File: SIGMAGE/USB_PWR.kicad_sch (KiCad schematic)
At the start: 45 parts, among them J1 UJ31CHG2SMTTR, U1 MAX8902BATA/V+T, U2 MAX8902BATA/V+T, U3 MAX8902BATA/V+T

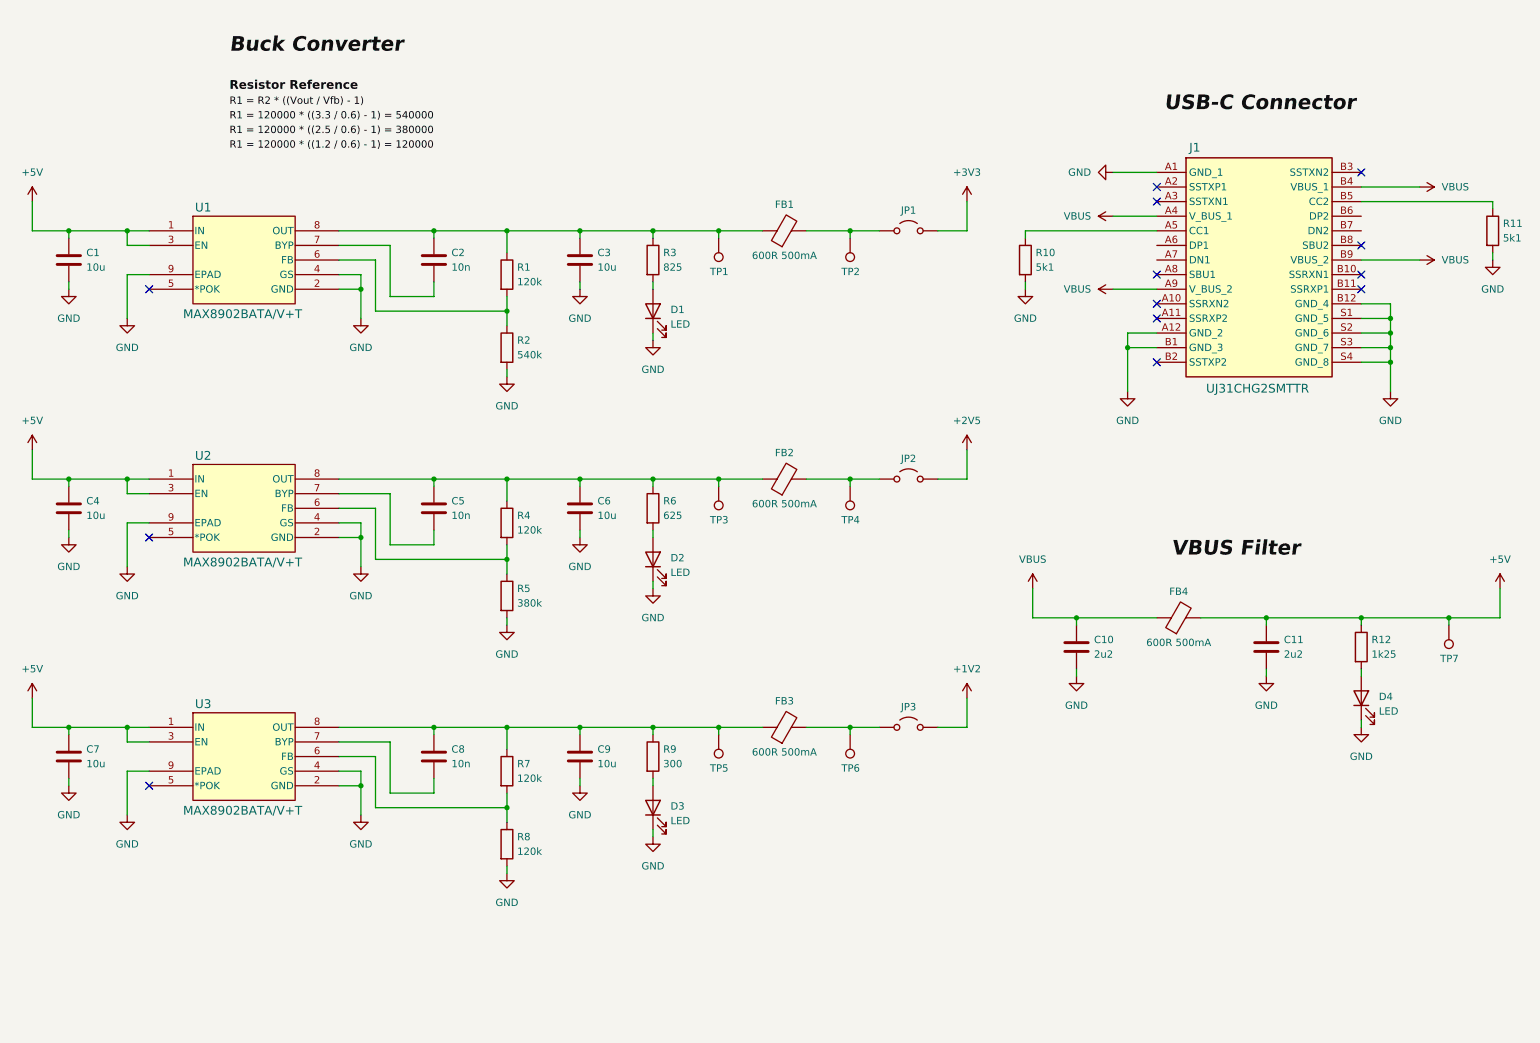
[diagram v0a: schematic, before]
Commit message: Finished schematic
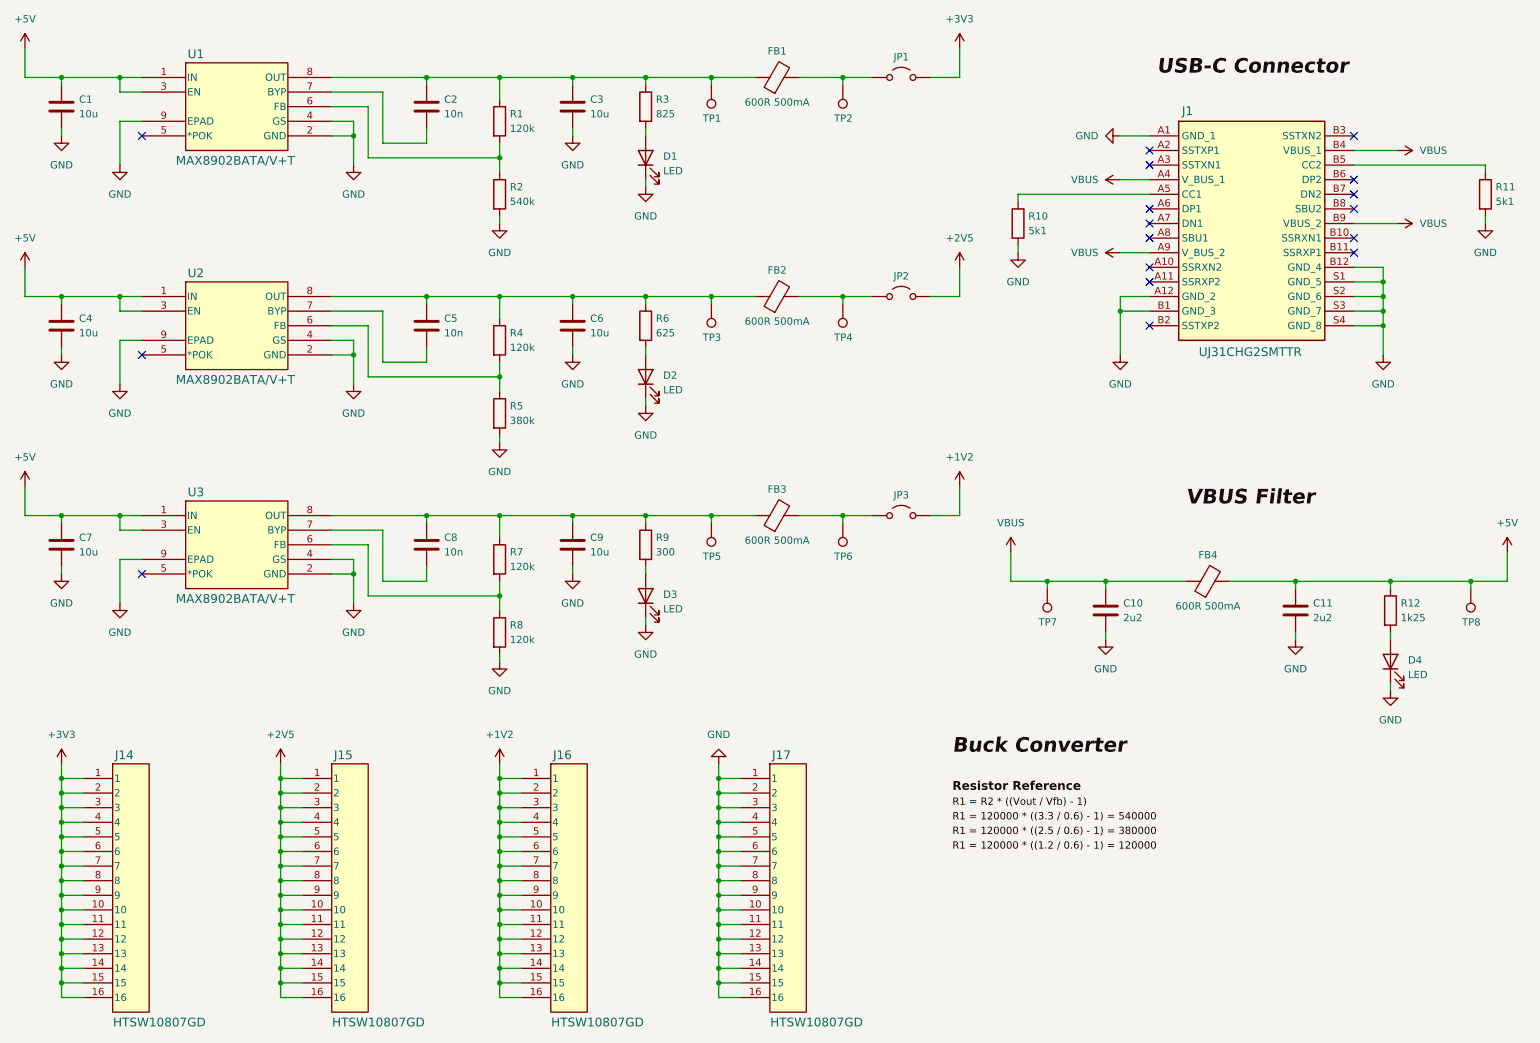
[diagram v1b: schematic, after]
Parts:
- added J14, J15, J16, J17: HTSW10807GD, SIGMAGE:HTSW10807GD, symbol SIGMAGE:HTSW10807GD
- added TP8: 3V3, symbol Connector:TestPoint
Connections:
- net +1V2: now also J16.1, J16.10, J16.11, J16.12, J16.13, J16.14, J16.15, J16.16, J16.2, J16.3, J16.4, J16.5, J16.6, J16.7, J16.8, J16.9
- net +2V5: now also J15.1, J15.10, J15.11, J15.12, J15.13, J15.14, J15.15, J15.16, J15.2, J15.3, J15.4, J15.5, J15.6, J15.7, J15.8, J15.9
- net +3V3: now also J14.1, J14.10, J14.11, J14.12, J14.13, J14.14, J14.15, J14.16, J14.2, J14.3, J14.4, J14.5, J14.6, J14.7, J14.8, J14.9
- net +5V: now also TP8.1; no longer TP7.1
- net GND: now also J17.1, J17.10, J17.11, J17.12, J17.13, J17.14, J17.15, J17.16, J17.2, J17.3, J17.4, J17.5, J17.6, J17.7, J17.8, J17.9
- net VBUS: now also TP7.1
- no-connect marks 13 -> 17
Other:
- moved on the sheet: C1, C10, C11, C2, C3, C4, C5, C6, C7, C8, C9, D1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
